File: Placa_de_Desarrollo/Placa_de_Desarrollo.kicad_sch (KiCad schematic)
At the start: 54 parts, among them J1 SD_Card, J10 5V_OUT, J11 3.3V_OUT, J12 ADC_VREF, J13 GND, J14 AGND, J15 VSYS_ALIMEANTACION_EXTERNA, J16 3V3_EN, J17 DEVICE I2C0, J18 PINES GPIO, J2 USB_B_Micro, J3 DEVICE I2C0, J4 GND, J5 GND, J6 GND, J7 GND, J8 GND, J9 GND, U1 Pico, U2 LM317_TO-220

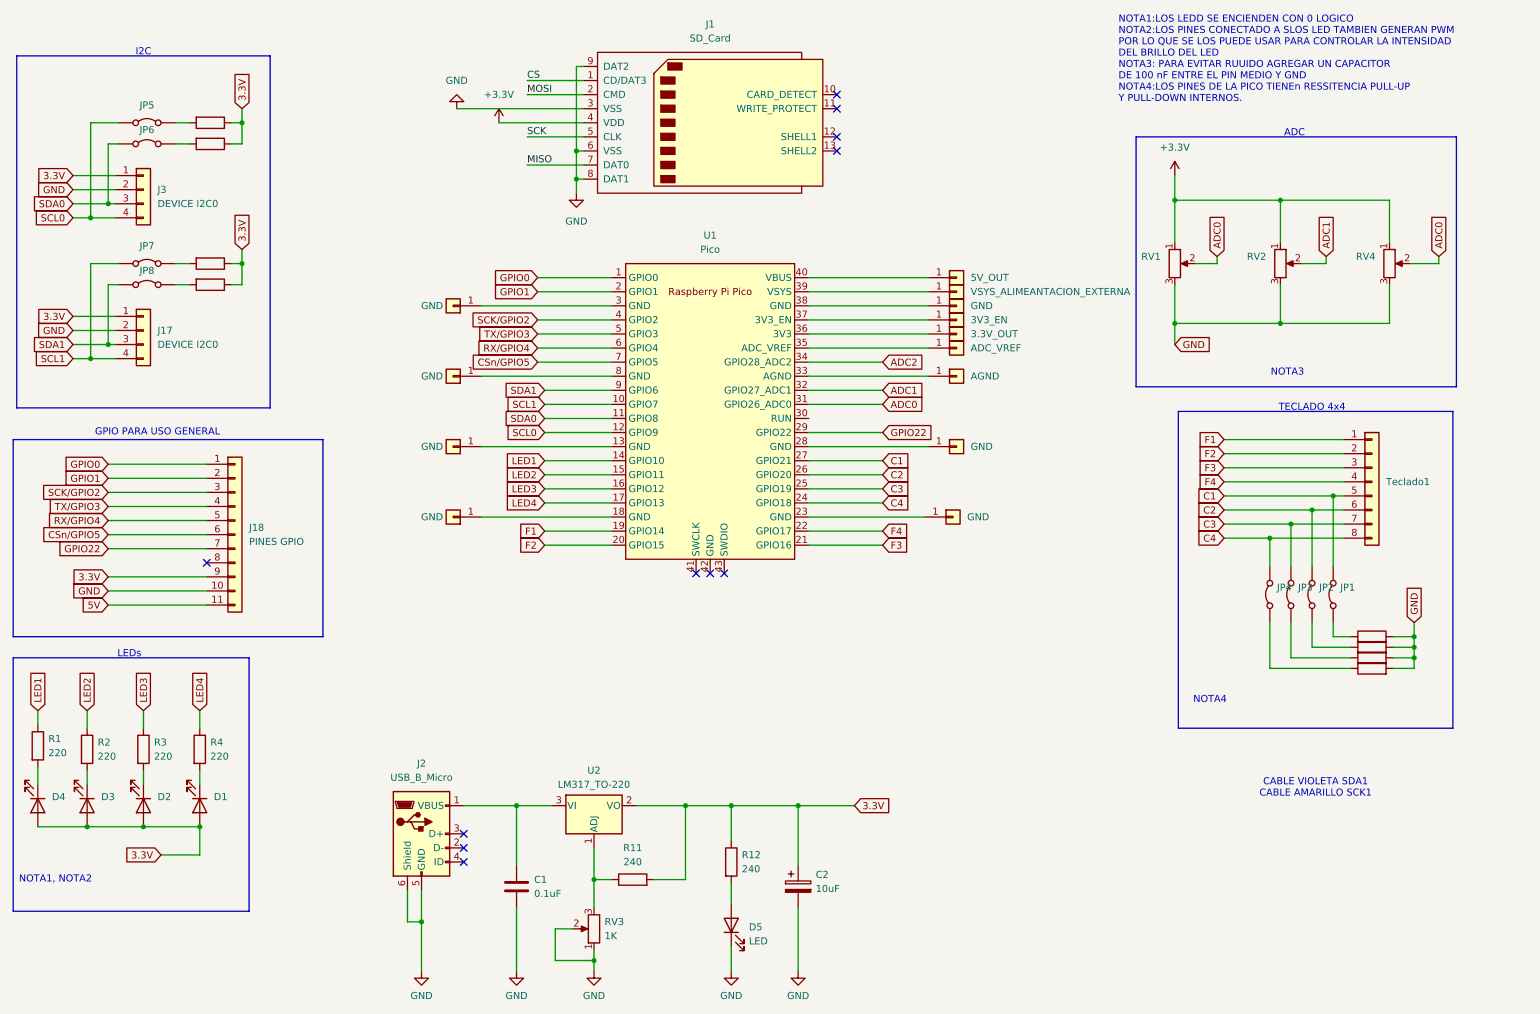
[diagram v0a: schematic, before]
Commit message: Placa_de_Desarrollo_7_6_2025
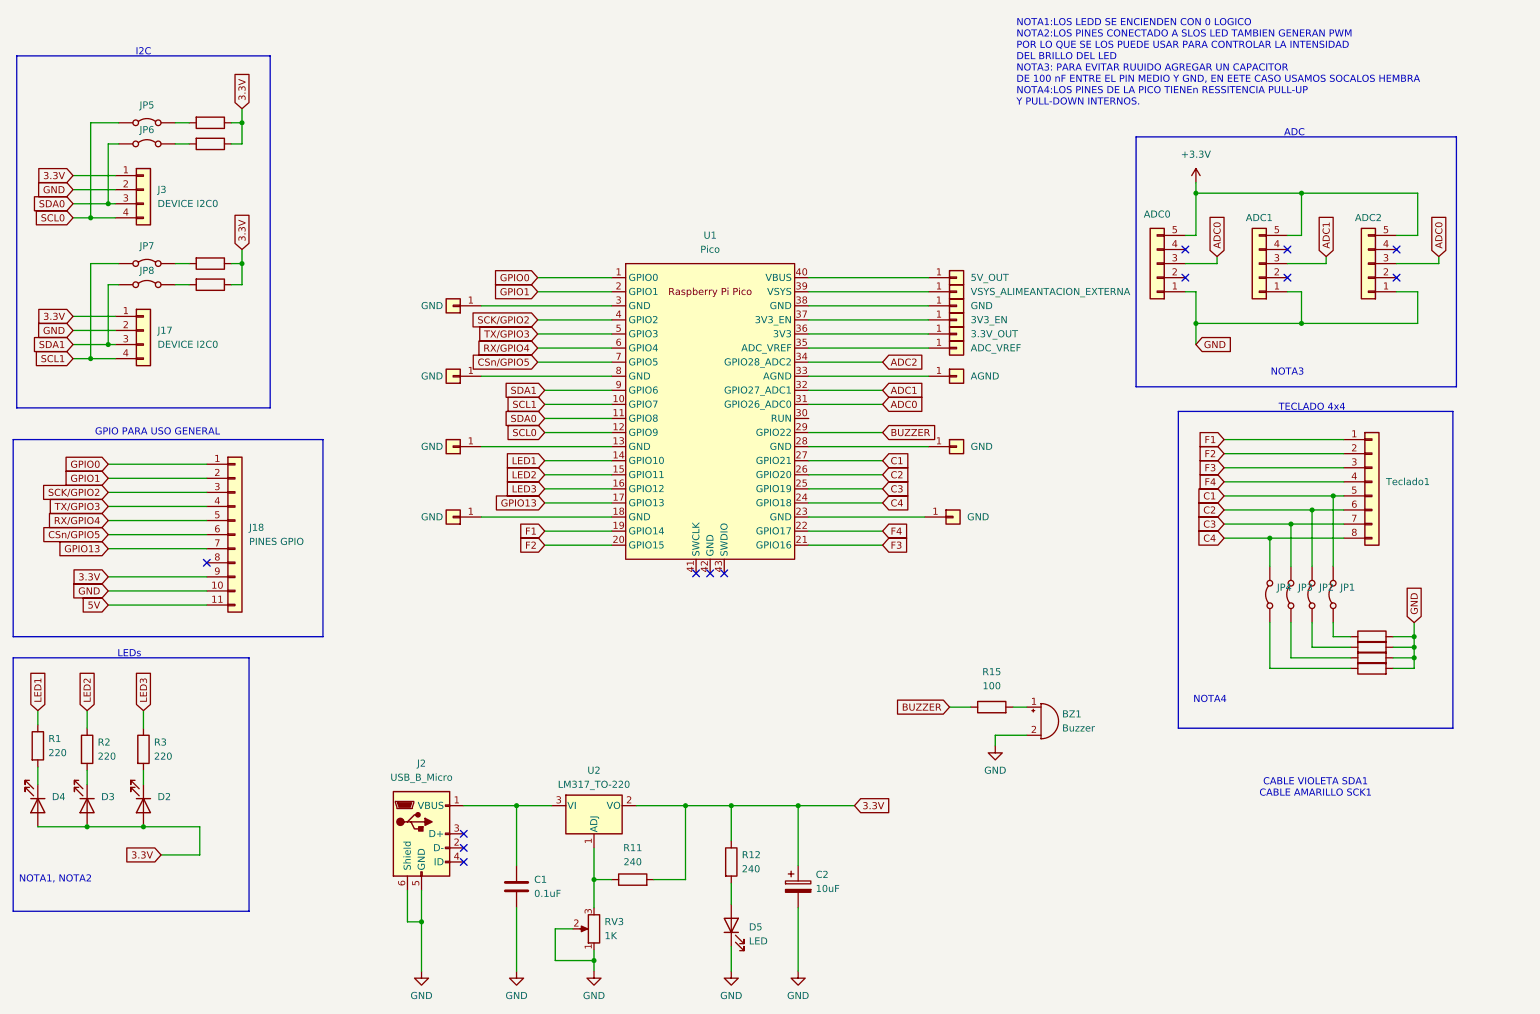
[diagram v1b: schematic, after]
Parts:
- removed D1: LED, symbol Device:LED
- removed J1: SD_Card, symbol Connector:SD_Card
- removed R4: 220, symbol Device:R
- removed RV1, RV2, RV4: R_Potentiometer, symbol Device:R_Potentiometer
- added BZ1: Buzzer, symbol Device:Buzzer
- added J19: ADC1, symbol Connector_Generic:Conn_01x05
- added J20: ADC2, symbol Connector_Generic:Conn_01x05
- added J21: ADC0, symbol Connector_Generic:Conn_01x05
- added R15: 100, symbol Device:R
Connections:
- net +3.3V: now also J19.5 (Pin_5), J20.5 (Pin_5), J21.5 (Pin_5)
- net ADC0: now also J20.3 (Pin_3), J21.3 (Pin_3)
- net ADC1: now also J19.3 (Pin_3)
- net GND: now also BZ1.2 (-), J19.1 (Pin_1), J20.1 (Pin_1), J21.1 (Pin_1)
- net GPIO22 renamed BUZZER
- net BUZZER: now also R15.1; no longer J18.7 (Pin_7)
- net LED4 renamed GPIO13
- net GPIO13: now also J18.7 (Pin_7)
- new net: BZ1.1 (+), R15.2
- no-connect marks 11 -> 13
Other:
- note added: "NOTA1:LOS LEDD SE ENCIENDEN CON 0 LOGICO NOTA2:LOS PINES CONECTADO A SLOS LED TAMBIEN GENERAN PWM POR LO QUE SE LOS PUEDE USAR PARA CONTROLAR LA INTENSIDAD DEL BRILLO DEL LED NOTA3: PARA EVITAR RUUIDO AGREGAR UN CAPACITOR DE 100 nF ENTRE EL PIN MEDIO Y GND, EN EETE CASO USAMOS SOCALOS HEMBRA NOTA4:LOS PINES DE LA PICO TIENEn RESSITENCIA PULL-UP Y PULL-DOWN INTERNOS."
- note removed: "NOTA1:LOS LEDD SE ENCIENDEN CON 0 LOGICO NOTA2:LOS PINES CONECTADO A SLOS LED TAMBIEN GENERAN PWM POR LO QUE SE LOS PUEDE USAR PARA CONTROLAR LA INTENSIDAD DEL BRILLO DEL LED NOTA3: PARA EVITAR RUUIDO AGREGAR UN CAPACITOR DE 100 nF ENTRE EL PIN MEDIO Y GND NOTA4:LOS PINES DE LA PICO TIENEn RESSITENCIA PULL-UP Y PULL-DOWN INTERNOS."
